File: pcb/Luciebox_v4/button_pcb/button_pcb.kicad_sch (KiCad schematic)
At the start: 67 parts, among them T1 terminal_8x1, T2 terminal_8x1

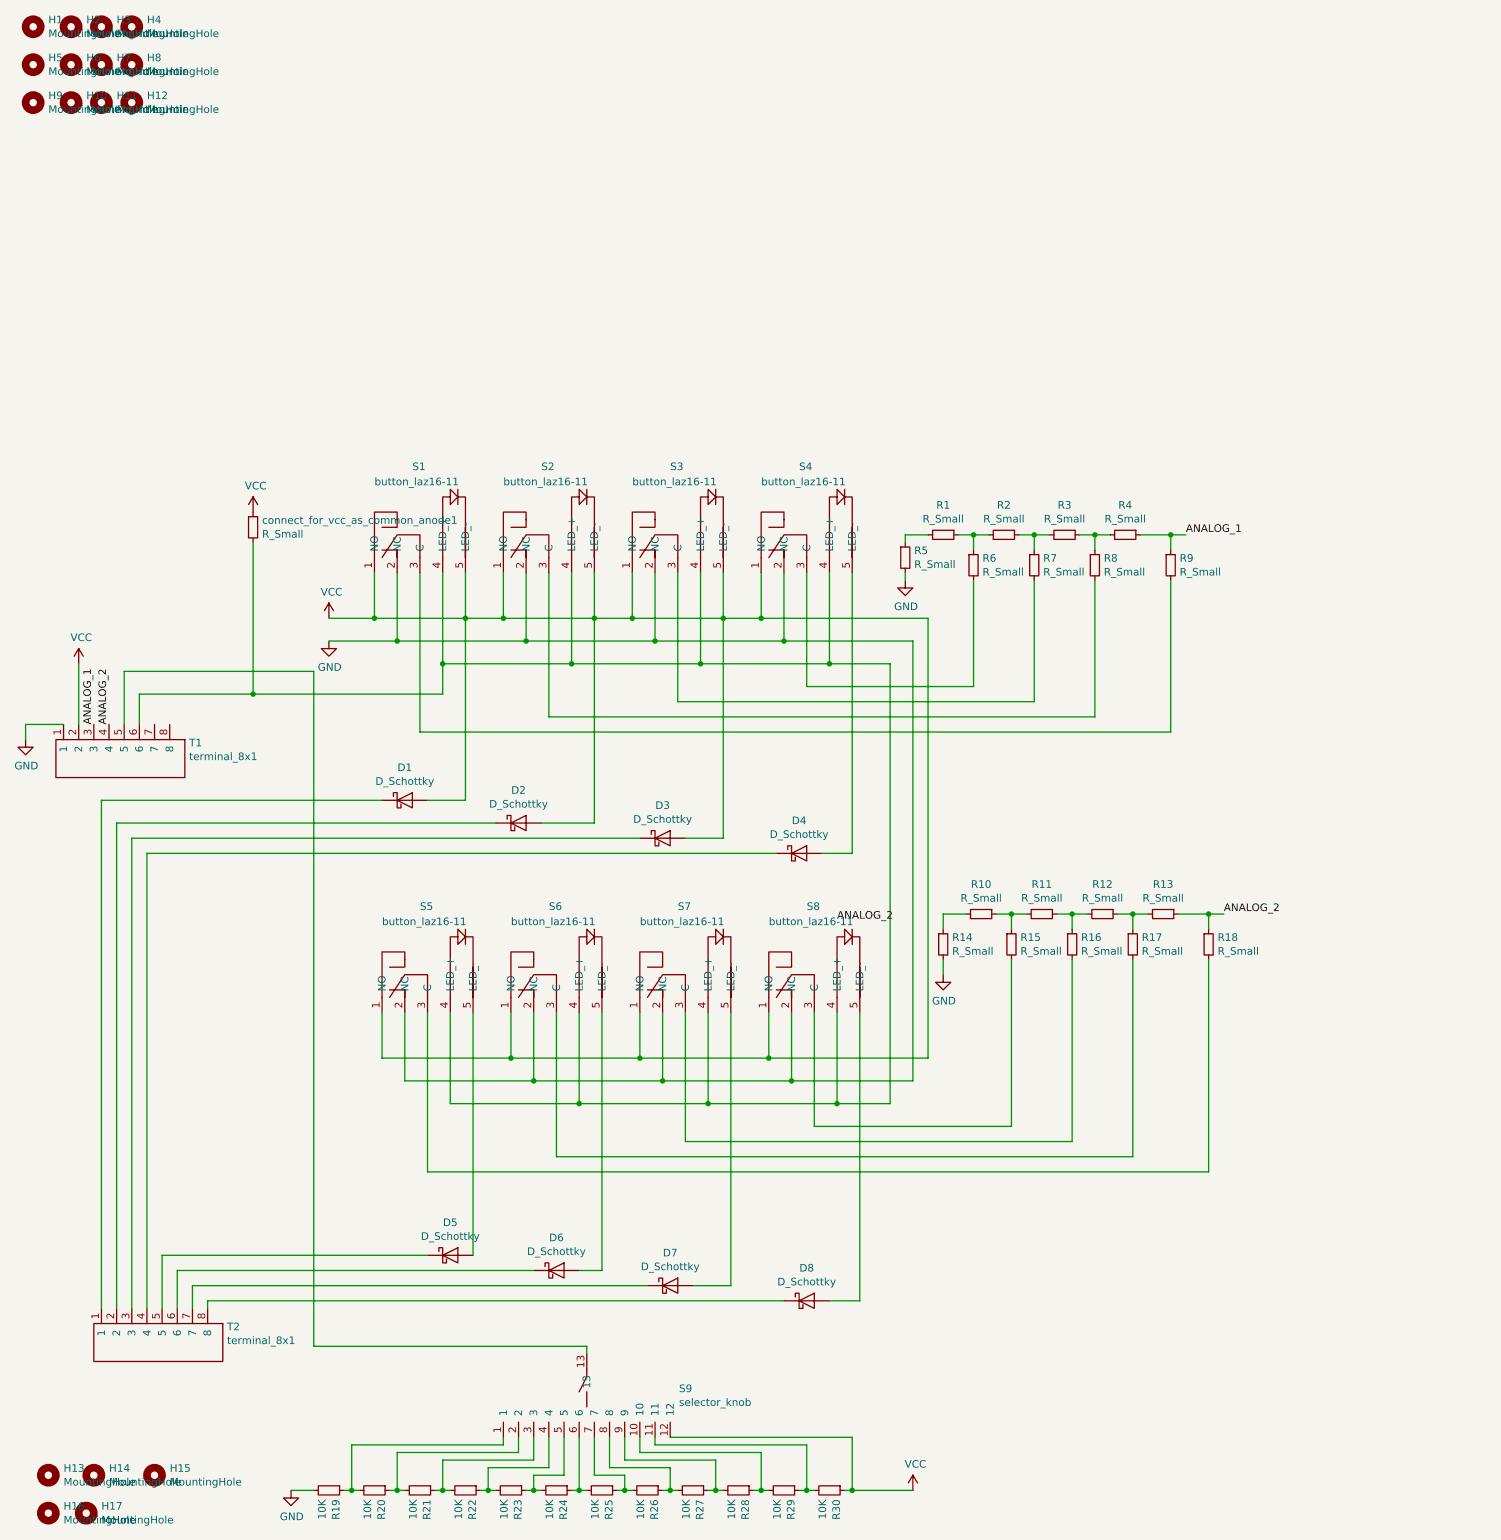
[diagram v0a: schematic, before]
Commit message: V4 main pcb ready for layouting
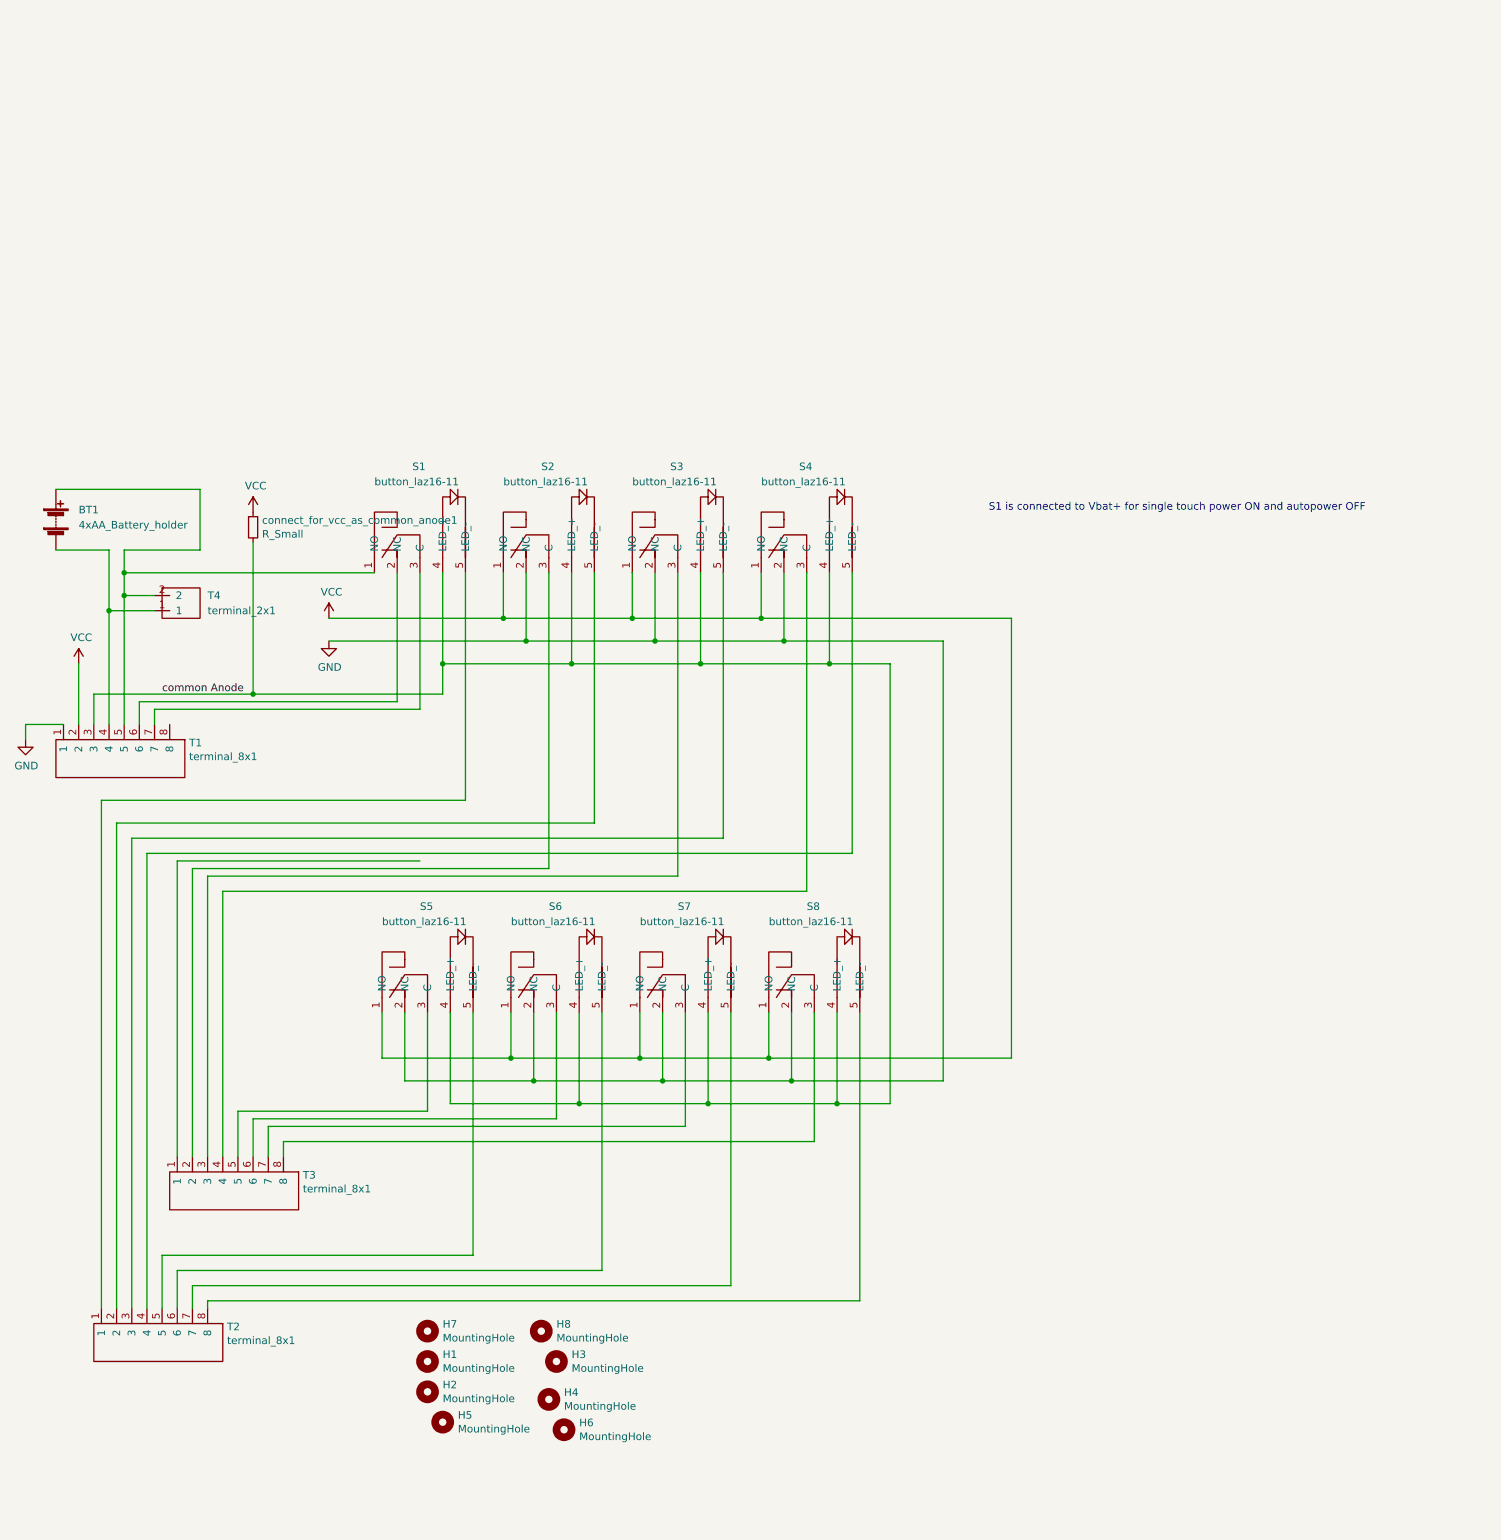
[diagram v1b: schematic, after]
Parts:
- removed D1, D2, D3, D4, D5, D6, D7, D8: D_Schottky, Luciebox_components:smd_throughhole_2_pins, symbol Luciebox_components:D_Schottky
- removed H1, H10, H12, H14, H15, H17, H7, H8, H9: MountingHole, Luciebox_components:MountingHole_4.3mm_M4, symbol Luciebox_components:MountingHole
- removed R1, R10, R11, R12, R13, R14, R15, R16, R17, R18, R2, R3, R4, R5, R6, R7, R8, R9: R_Small, Luciebox_components:1206_0805, symbol Luciebox_components:R_Small
- removed R19, R20, R21, R22, R23, R24, R25, R26, R27, R28, R29, R30: 10K, Luciebox_components:1206_0805, symbol Luciebox_components:R_Small-Device
- removed S9: selector_knob, Luciebox_components:Rotary_Switch, symbol Luciebox_components:selector_knob
- added BT1: 4xAA_Battery_holder, Luciebox_components:BatteryHolder_4xAA, symbol Luciebox_components:4xAA_Battery_holder
- added T3: terminal_8x1, Luciebox_components:Terminal_8x1_100mil, symbol Luciebox_components:terminal_8x1
- added T4: terminal_2x1, Luciebox_components:Terminal_2x1_100mil, symbol Luciebox_components:terminal_2x1
- S1, S2, S3, S4, S5, S6, S7, S8: footprint Luciebox_components:button_LAZ16-11 -> Luciebox_components:button_LAZ16-11_big_holes
- renumbered H16 to H1, H6 to H2, H13 to H3, H11 to H4, H3 to H6, H2 to H7, H4 to H8
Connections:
- net ANALOG_1 is gone; now on net common Anode: T1.3
- net GND: no longer S1.2 (NC)
- net VCC: no longer S1.1 (NO), S1.5 (LED_-), S2.5 (LED_-), S3.5 (LED_-)
- net at T2.8: now also S8.5 (LED_-)
- net at S4.3 (C): now also T3.4
- net at S1.3 (C): now also T1.7
- net common Anode: now reaches S1.4 (LED_+), S2.4 (LED_+), S3.4 (LED_+), S4.4 (LED_+), S5.4 (LED_+), S6.4 (LED_+), S7.4 (LED_+), S8.4 (LED_+), connect_for_vcc_as_common_anode1.2
- net common Anode: no longer T1.6
- net at T2.4: now also S4.5 (LED_-)
- net at S8.3 (C): now also T3.8
- net at S3.3 (C): now also T3.3
- net at T2.5: now also S5.5 (LED_-)
- net at S6.3 (C): now also T3.6
- net at S2.3 (C): now also T3.2
- net at S6.5 (LED_-): now also T2.6
- net at T1.5: now also S1.1 (NO), BT1.1 (+), T4.2
- net at T2.2: now also S2.5 (LED_-)
- net at T2.1: now also S1.5 (LED_-)
- net at T2.3: now also S3.5 (LED_-)
- net at T2.7: now also S7.5 (LED_-)
- net at S7.3 (C): now also T3.7
- net at S5.3 (C): now also T3.5
- net ANALOG_2: no longer names the net of T1.4
- net ANALOG_2: now also BT1.2 (-), T4.1
- new net: S1.2 (NC), T1.6
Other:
- note added: "S1 is connected to Vbat+ for single touch power ON and autopower OFF"
- moved on the sheet: H1, H2, H3, H4, H5, H6, H7, H8
